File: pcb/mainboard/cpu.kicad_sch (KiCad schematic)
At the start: 11 parts, among them U101 RP-A311D

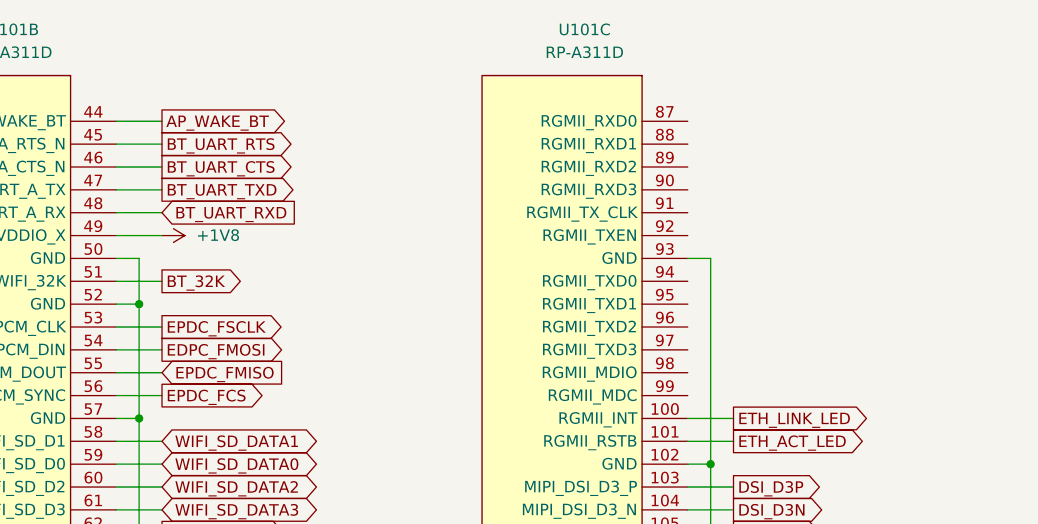
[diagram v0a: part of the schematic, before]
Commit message: pcb: r0.1 mb routing done
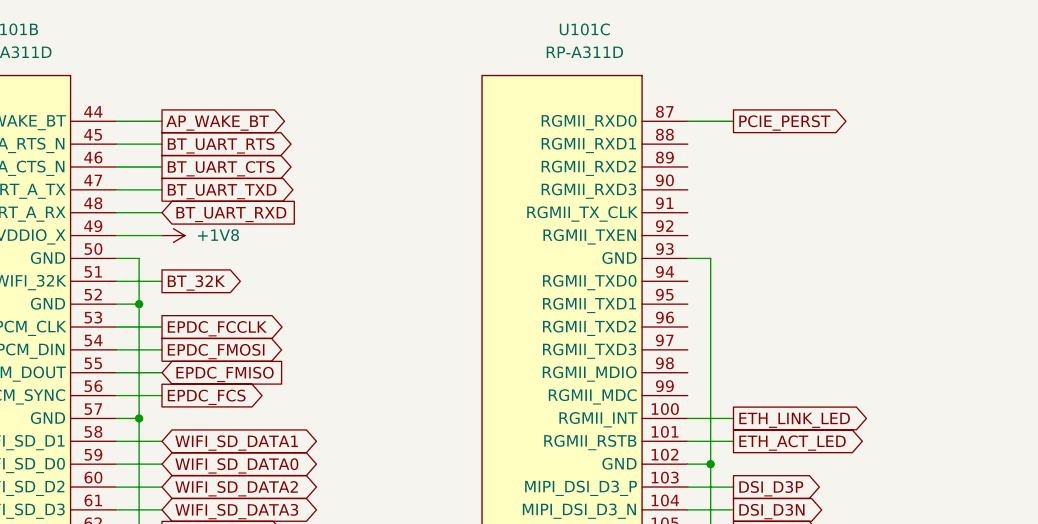
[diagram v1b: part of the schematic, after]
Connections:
- net PCIE_PERST: now reaches U101.87 (RGMII_RXD0)
- net EDPC_FMOSI renamed EPDC_FMOSI
- net EPDC_FSCLK renamed EPDC_FCCLK
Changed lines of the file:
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@@
+    (stroke (width 0) (type default) (color 0 0 0 0))
+  )
+  (wire (pts (xy 180.34 45.72) (xy 185.42 45.72))
     (stroke (width 0) (type default) (color 0 0 0 0))
   )
@@
     )
   )
-  (global_label "EPDC_FSCLK" (shape output) (at 121.92 68.58 0) (fields_autoplaced)
-    (effects (font (size 1.27 1.27)) (justify left))
-    (property "Intersheet References" "${INTERSHEET_REFS}" (id 0) (at 136.126 68.5006 0)
-      (effects (font (size 1.27 1.27)) (justify left) hide)
-    )
-  )
-  (global_label "EDPC_FMOSI" (shape output) (at 121.92 71.12 0) (fields_autoplaced)
+  (global_label "EPDC_FCCLK" (shape output) (at 121.92 68.58 0) (fields_autoplaced)
+    (effects (font (size 1.27 1.27)) (justify left))
+    (property "Intersheet References" "${INTERSHEET_REFS}" (id 0) (at 136.1864 68.5006 0)
+      (effects (font (size 1.27 1.27)) (justify left) hide)
+    )
+  )
+  (global_label "EPDC_FMOSI" (shape output) (at 121.92 71.12 0) (fields_autoplaced)
     (effects (font (size 1.27 1.27)) (justify left))
     (property "Intersheet References" "${INTERSHEET_REFS}" (id 0) (at 135.9445 71.0406 0)
@@
       (effects (font (size 1.27 1.27)) (justify left) hide)
     )
+  )
+  (global_label "PCIE_PERST" (shape output) (at 185.42 45.72 0) (fields_autoplaced)
+    (effects (font (size 1.27 1.27)) (justify left))
+    (property "Intersheet References" "${INTERSHEET_REFS}" (id 0) (at 198.9607 45.6406 0)
+      (effects (font (size 1.27 1.27)) (justify left) hide)
+    )
